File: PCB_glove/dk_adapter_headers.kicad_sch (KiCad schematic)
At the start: 1 part, among them J1 STM32N6570-DK LOGICAL ADAPTER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

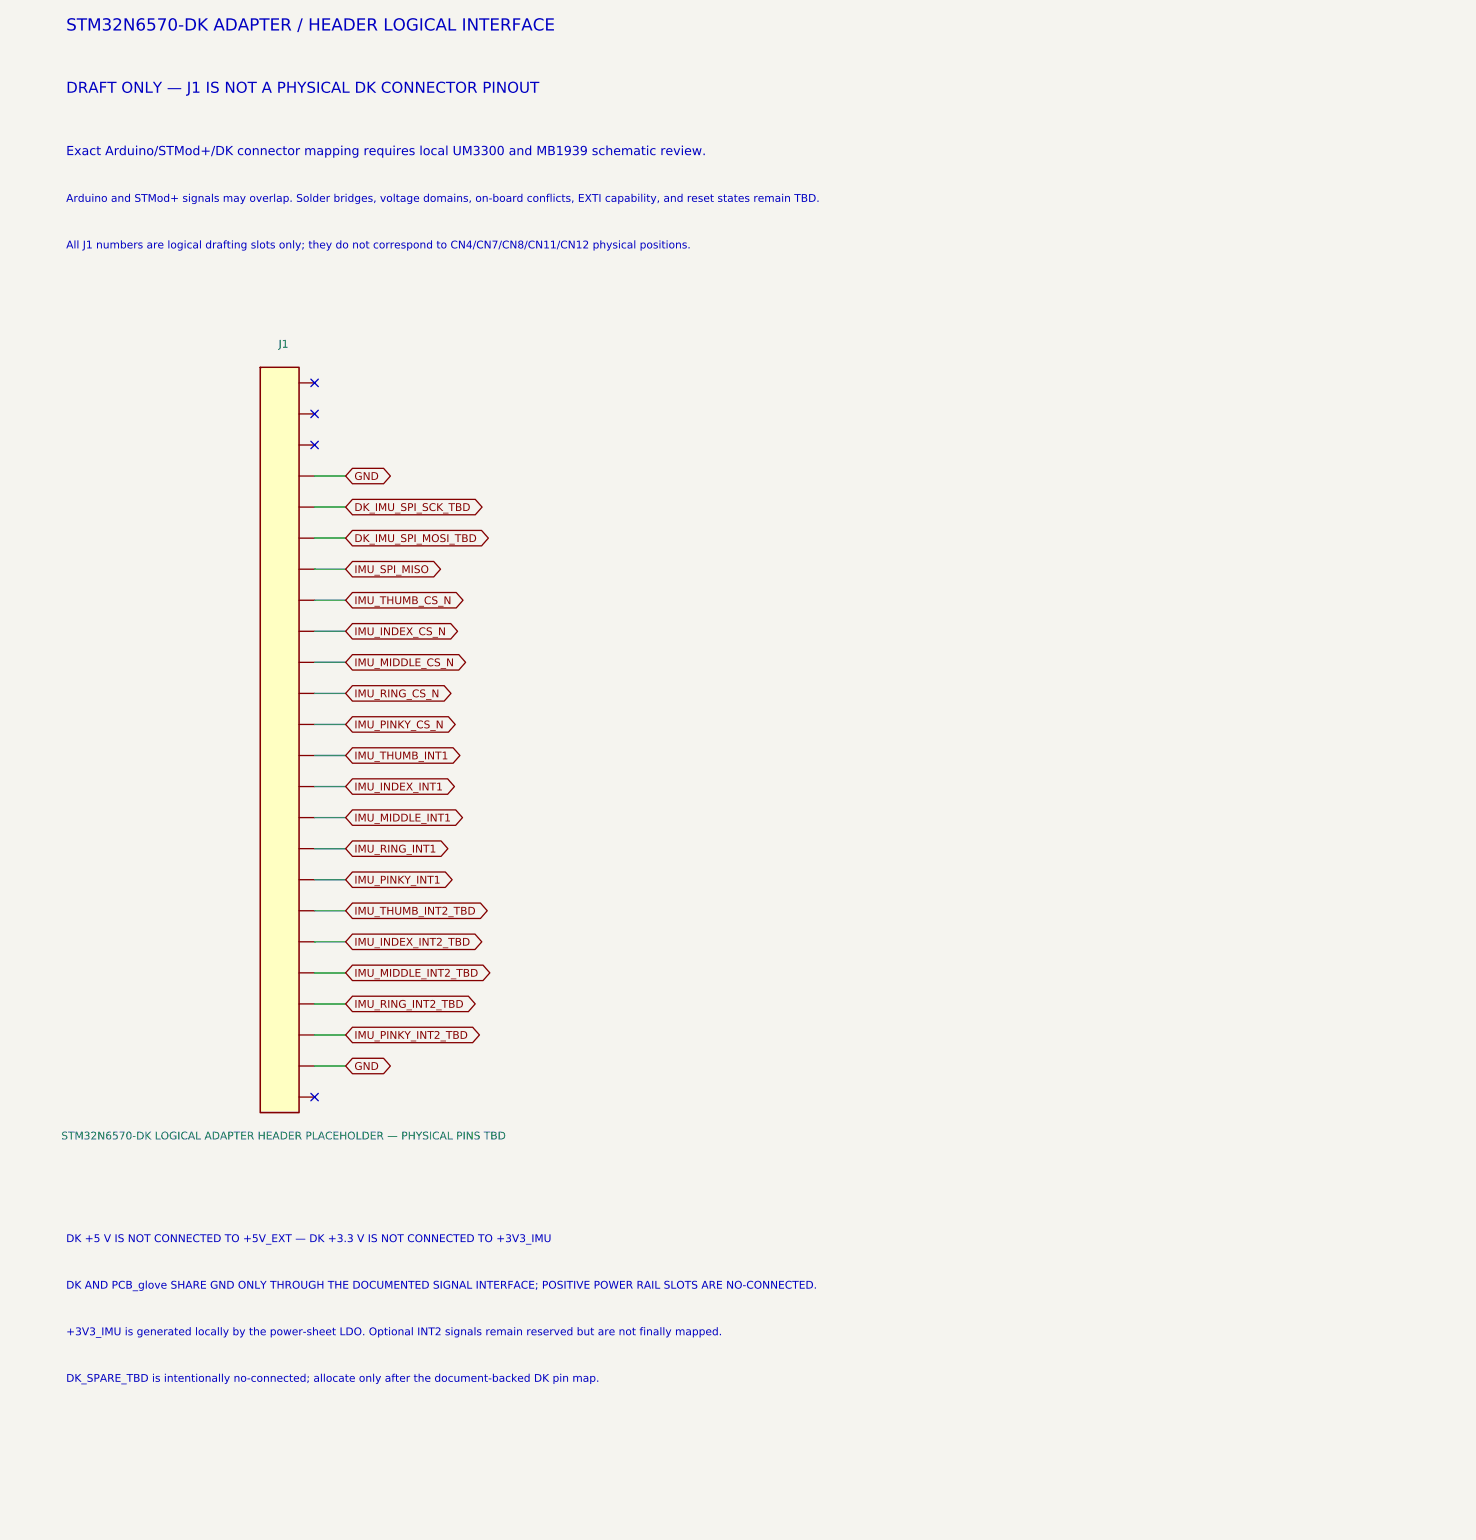
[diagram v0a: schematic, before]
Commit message: all
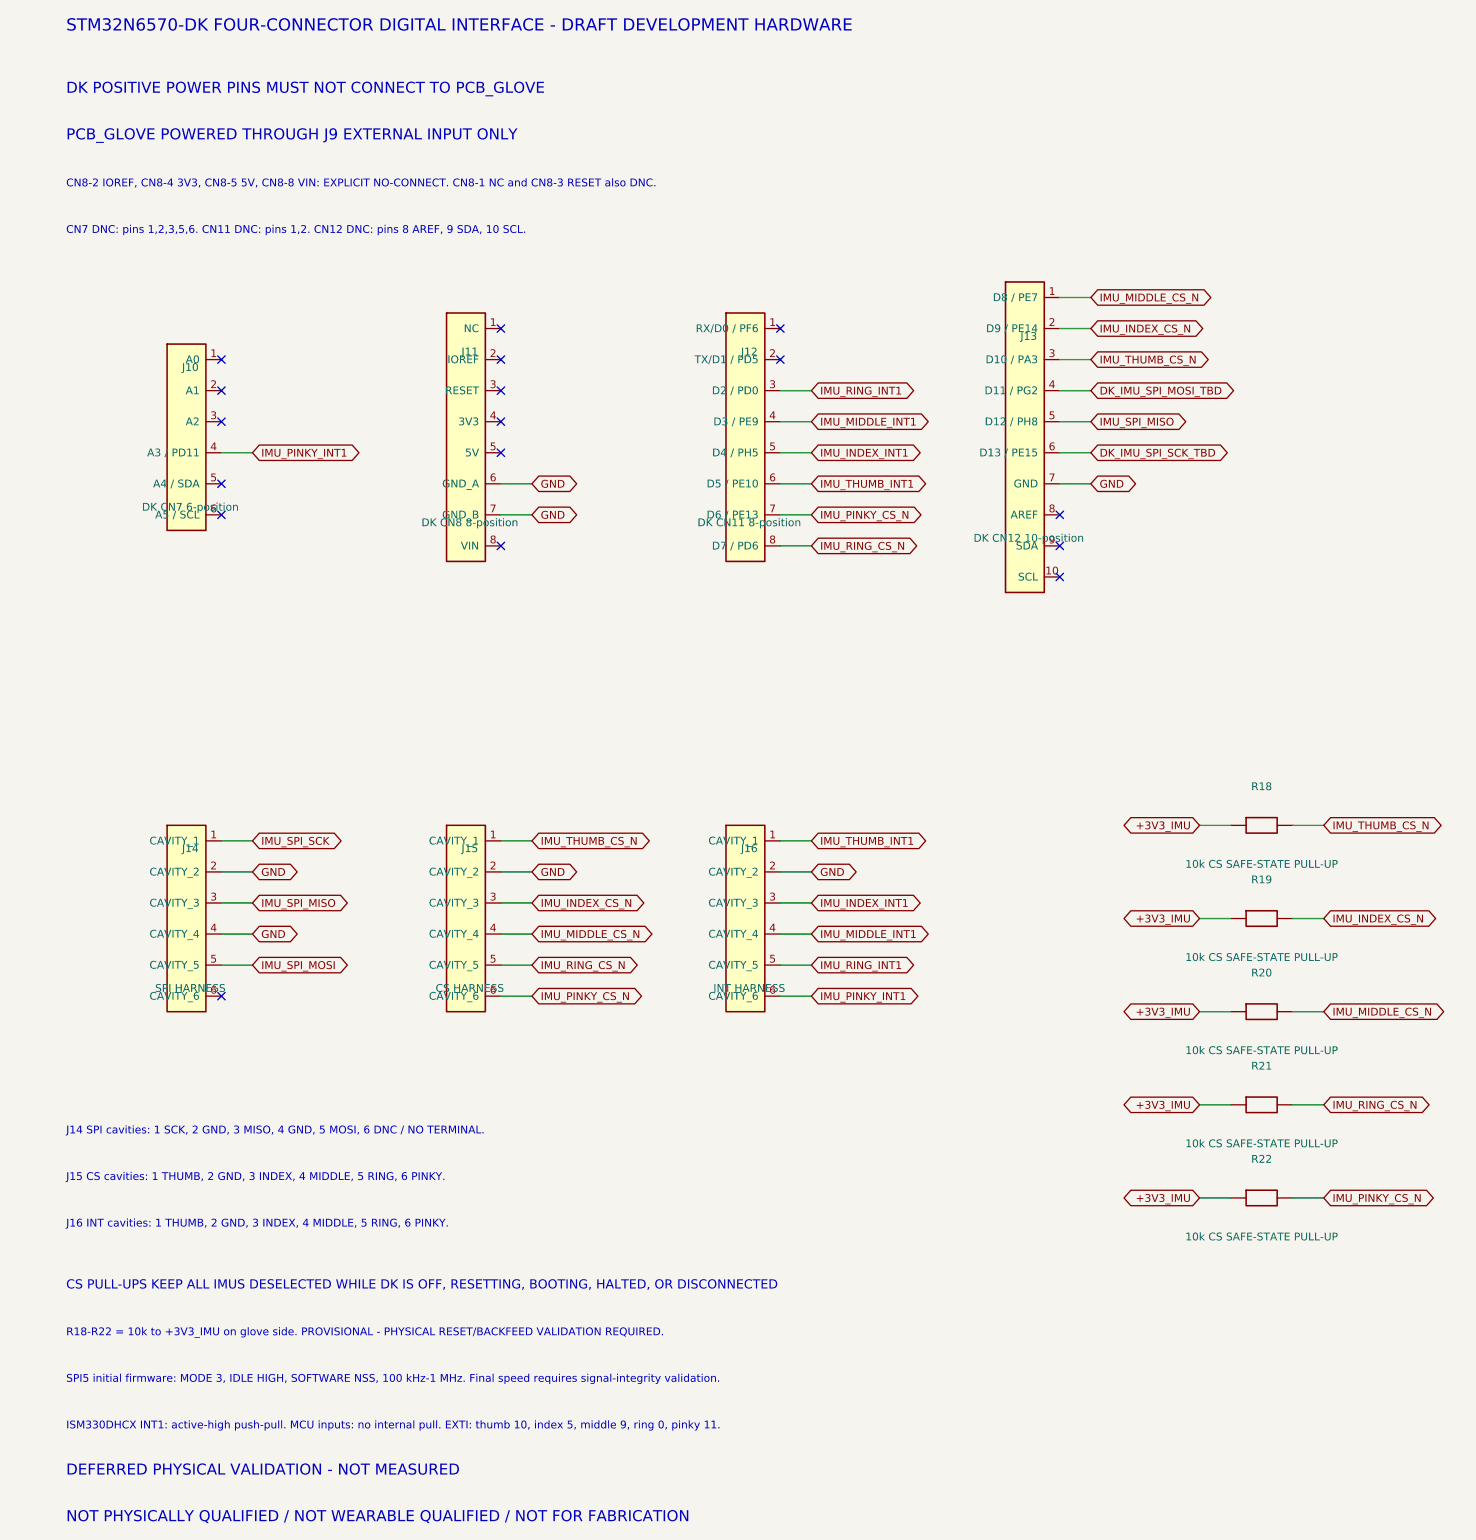
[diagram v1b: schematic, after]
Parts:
- removed J1: STM32N6570-DK LOGICAL ADAPTER HEADER PLACEHOLDER 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, symbol PCB_glove_Draft:DK_LOGICAL_24
- added J10: DK CN7 6-position, symbol PCB_glove_Draft:DK_CN7_6
- added J11: DK CN8 8-position, symbol PCB_glove_Draft:DK_CN8_8
- added J12: DK CN11 8-position, symbol PCB_glove_Draft:DK_CN11_8
- added J13: DK CN12 10-position, symbol PCB_glove_Draft:DK_CN12_10
- added J14: SPI HARNESS, symbol PCB_glove_Draft:HARNESS_1X6
- added J15: CS HARNESS, symbol PCB_glove_Draft:HARNESS_1X6
- added J16: INT HARNESS, symbol PCB_glove_Draft:HARNESS_1X6
- added R18, R19, R20, R21, R22: 10k CS SAFE-STATE PULL-UP, Resistor_SMD:R_0603_1608Metric, symbol PCB_glove_Draft:R_OPTION
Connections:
- net DK_IMU_SPI_MOSI_TBD: now also J13.4 (D11 / PG2)
- net DK_IMU_SPI_SCK_TBD: now also J13.6 (D13 / PE15)
- net GND: now also J11.6 (GND_A), J11.7 (GND_B), J13.7 (GND), J14.2 (CAVITY_2), J14.4 (CAVITY_4), J15.2 (CAVITY_2), J16.2 (CAVITY_2)
- net IMU_INDEX_CS_N: now also J13.2 (D9 / PE14), J15.3 (CAVITY_3), R19.2
- net IMU_INDEX_INT1: now also J12.5 (D4 / PH5), J16.3 (CAVITY_3)
- net IMU_MIDDLE_CS_N: now also J13.1 (D8 / PE7), J15.4 (CAVITY_4), R20.2
- net IMU_MIDDLE_INT1: now also J12.4 (D3 / PE9), J16.4 (CAVITY_4)
- net IMU_PINKY_CS_N: now also J12.7 (D6 / PE13), J15.6 (CAVITY_6), R22.2
- net IMU_PINKY_INT1: now also J10.4 (A3 / PD11), J16.6 (CAVITY_6)
- net IMU_RING_CS_N: now also J12.8 (D7 / PD6), J15.5 (CAVITY_5), R21.2
- net IMU_RING_INT1: now also J12.3 (D2 / PD0), J16.5 (CAVITY_5)
- net IMU_SPI_MISO: now also J13.5 (D12 / PH8), J14.3 (CAVITY_3)
- net IMU_THUMB_CS_N: now also J13.3 (D10 / PA3), J15.1 (CAVITY_1), R18.2
- net IMU_THUMB_INT1: now also J12.6 (D5 / PE10), J16.1 (CAVITY_1)
- new net +3V3_IMU: R18.1, R19.1, R20.1, R21.1, R22.1
- new net IMU_SPI_MOSI: J14.5 (CAVITY_5)
- new net IMU_SPI_SCK: J14.1 (CAVITY_1)
- no-connect marks 4 -> 17
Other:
- note added: "CN7 DNC: pins 1,2,3,5,6. CN11 DNC: pins 1,2. CN12 DNC: pins 8 AREF, 9 SDA, 10 SCL."
- note added: "CN8-2 IOREF, CN8-4 3V3, CN8-5 5V, CN8-8 VIN: EXPLICIT NO-CONNECT. CN8-1 NC and CN8-3 RESET also DNC."
- note added: "CS PULL-UPS KEEP ALL IMUS DESELECTED WHILE DK IS OFF, RESETTING, BOOTING, HALTED, OR DISCONNECTED"
- note added: "DEFERRED PHYSICAL VALIDATION - NOT MEASURED"
- note added: "DK POSITIVE POWER PINS MUST NOT CONNECT TO PCB_GLOVE"
- note added: "ISM330DHCX INT1: active-high push-pull. MCU inputs: no internal pull. EXTI: thumb 10, index 5, middle 9, ring 0, pinky 11."
- note added: "J14 SPI cavities: 1 SCK, 2 GND, 3 MISO, 4 GND, 5 MOSI, 6 DNC / NO TERMINAL."
- note added: "J15 CS cavities: 1 THUMB, 2 GND, 3 INDEX, 4 MIDDLE, 5 RING, 6 PINKY."
- note added: "J16 INT cavities: 1 THUMB, 2 GND, 3 INDEX, 4 MIDDLE, 5 RING, 6 PINKY."
- note added: "NOT PHYSICALLY QUALIFIED / NOT WEARABLE QUALIFIED / NOT FOR FABRICATION"
- note added: "PCB_GLOVE POWERED THROUGH J9 EXTERNAL INPUT ONLY"
- note added: "R18-R22 = 10k to +3V3_IMU on glove side. PROVISIONAL - PHYSICAL RESET/BACKFEED VALIDATION REQUIRED."
- note added: "SPI5 initial firmware: MODE 3, IDLE HIGH, SOFTWARE NSS, 100 kHz-1 MHz. Final speed requires signal-integrity validation."
- note added: "STM32N6570-DK FOUR-CONNECTOR DIGITAL INTERFACE - DRAFT DEVELOPMENT HARDWARE"
- note removed: "+3V3_IMU is generated locally by the power-sheet LDO. Optional INT2 signals remain reserved but are not finally mapped."
- note removed: "All J1 numbers are logical drafting slots only; they do not correspond to CN4/CN7/CN8/CN11/CN12 physical positions."
- note removed: "Arduino and STMod+ signals may overlap. Solder bridges, voltage domains, on-board conflicts, EXTI capability, and reset states remain TBD."
- note removed: "DK +5 V IS NOT CONNECTED TO +5V_EXT — DK +3.3 V IS NOT CONNECTED TO +3V3_IMU"
- note removed: "DK AND PCB_glove SHARE GND ONLY THROUGH THE DOCUMENTED SIGNAL INTERFACE; POSITIVE POWER RAIL SLOTS ARE NO-CONNECTED."
- note removed: "DK_SPARE_TBD is intentionally no-connected; allocate only after the document-backed DK pin map."
- note removed: "DRAFT ONLY — J1 IS NOT A PHYSICAL DK CONNECTOR PINOUT"
- note removed: "Exact Arduino/STMod+/DK connector mapping requires local UM3300 and MB1939 schematic review."
- note removed: "STM32N6570-DK ADAPTER / HEADER LOGICAL INTERFACE"
